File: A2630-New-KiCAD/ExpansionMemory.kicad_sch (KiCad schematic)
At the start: 16 parts, among them U102 27C256, U103 27C256, U406 SDRAM_256Mb(16Mx16), U407 SDRAM_256Mb(16Mx16), U408 SDRAM_256Mb(16Mx16), U409 SDRAM_256Mb(16Mx16)

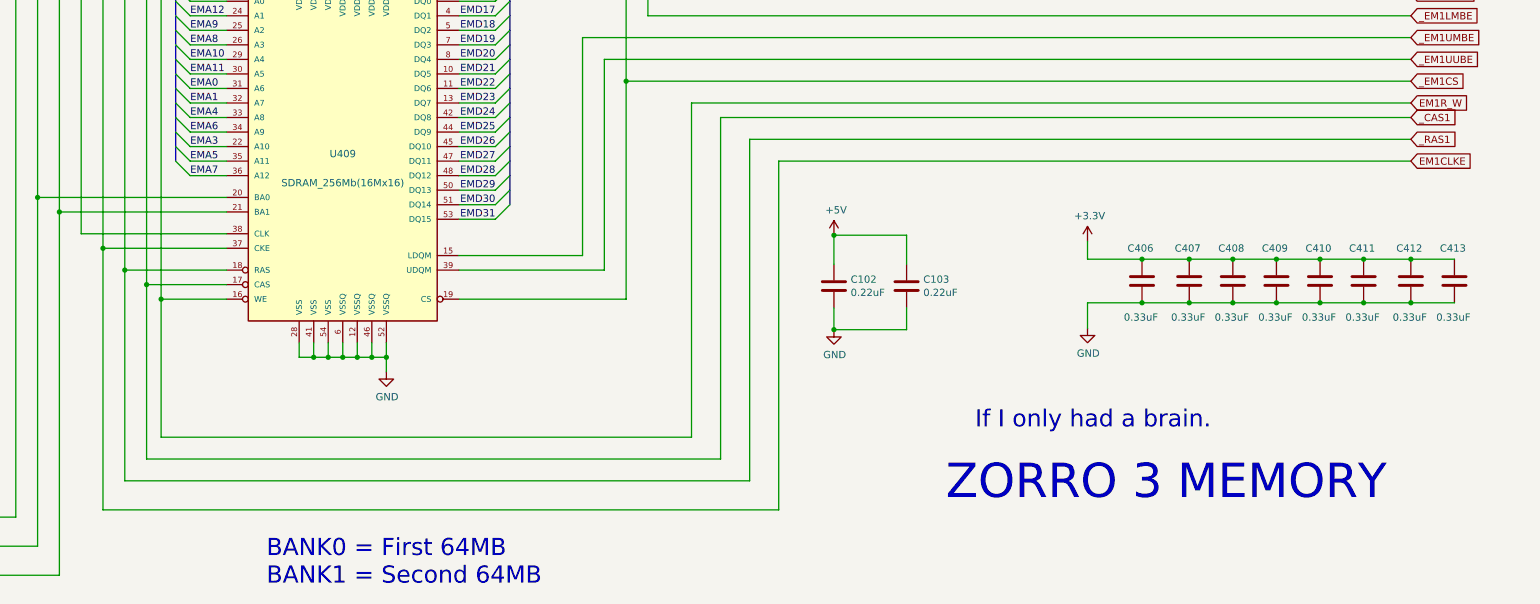
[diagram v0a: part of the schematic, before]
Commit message: Add files via upload
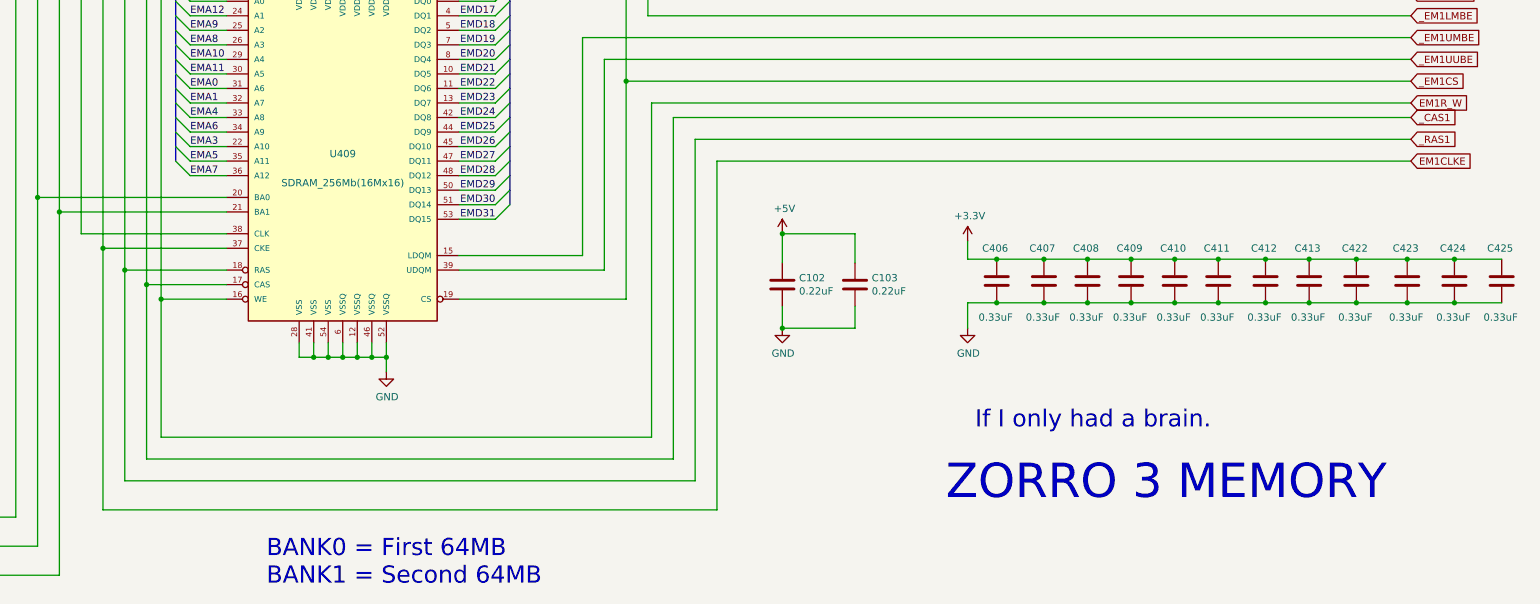
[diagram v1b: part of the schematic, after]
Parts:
- added C422, C423, C424, C425: 0.33uF, Capacitor_SMD:C_0805_2012Metric, symbol Device:C
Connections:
- net +3V3: now also C422.1, C423.1, C424.1, C425.1
- net GND: now also C422.2, C423.2, C424.2, C425.2
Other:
- moved on the sheet: C102, C103, C406, C407, C408, C409, C410, C411, C412, C413
